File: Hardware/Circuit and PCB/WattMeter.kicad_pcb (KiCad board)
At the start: 2 copper layers, 185 x 126.1 mm, 80 parts, among them IC1 ATM90E32AS-AU-R, IC2 LM2621MMX_NOPB, J1 LCD Pins, J10 I2 Use/GND, J11 Input, J12 V3 Use/GND, J13 I1, J14 Series/Para, J15 Series/Para, J16 V2 Use/GND, J17 V1, J18 VCC Pins, J19 Boost Input, J2 Button Pins, J3 GSD09002SEU, J4 Extras, J5 SPI ATM90, J9 I3 Use/GND, T1 CT1020, T4 10:1, U1 ESP32-C6-DEVKITC-1-N8, U3 PCF8523T/1_118, Y1 16.384MHz, Y2 32.768kHz

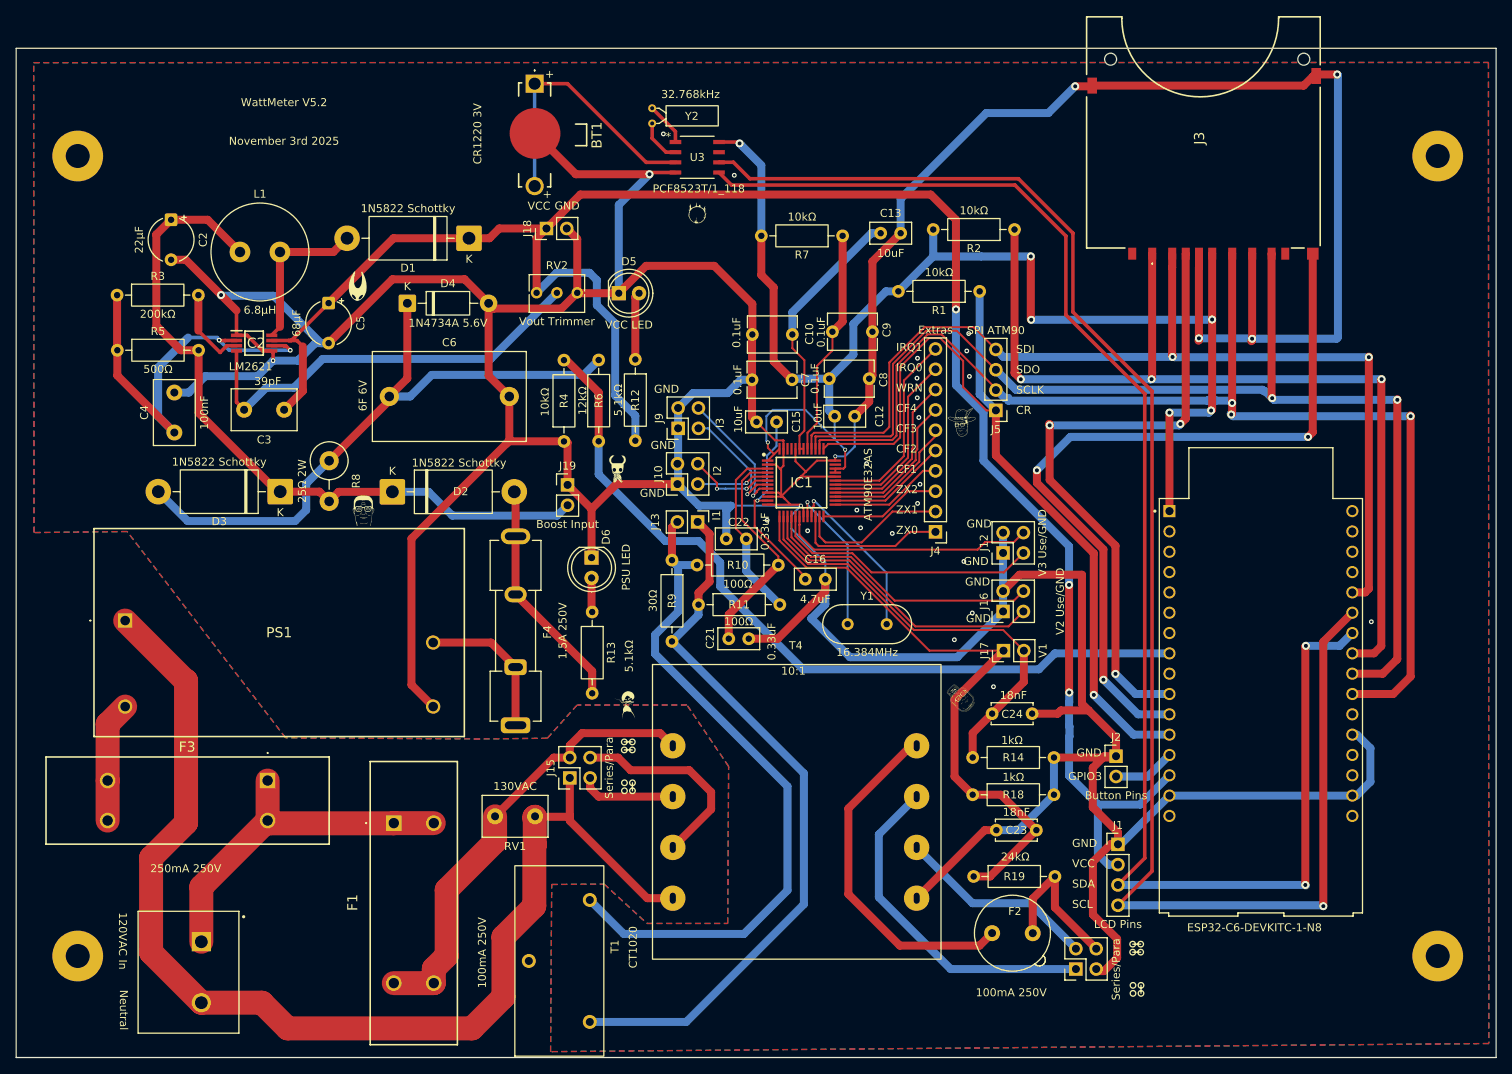
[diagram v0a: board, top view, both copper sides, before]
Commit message: Add some plots
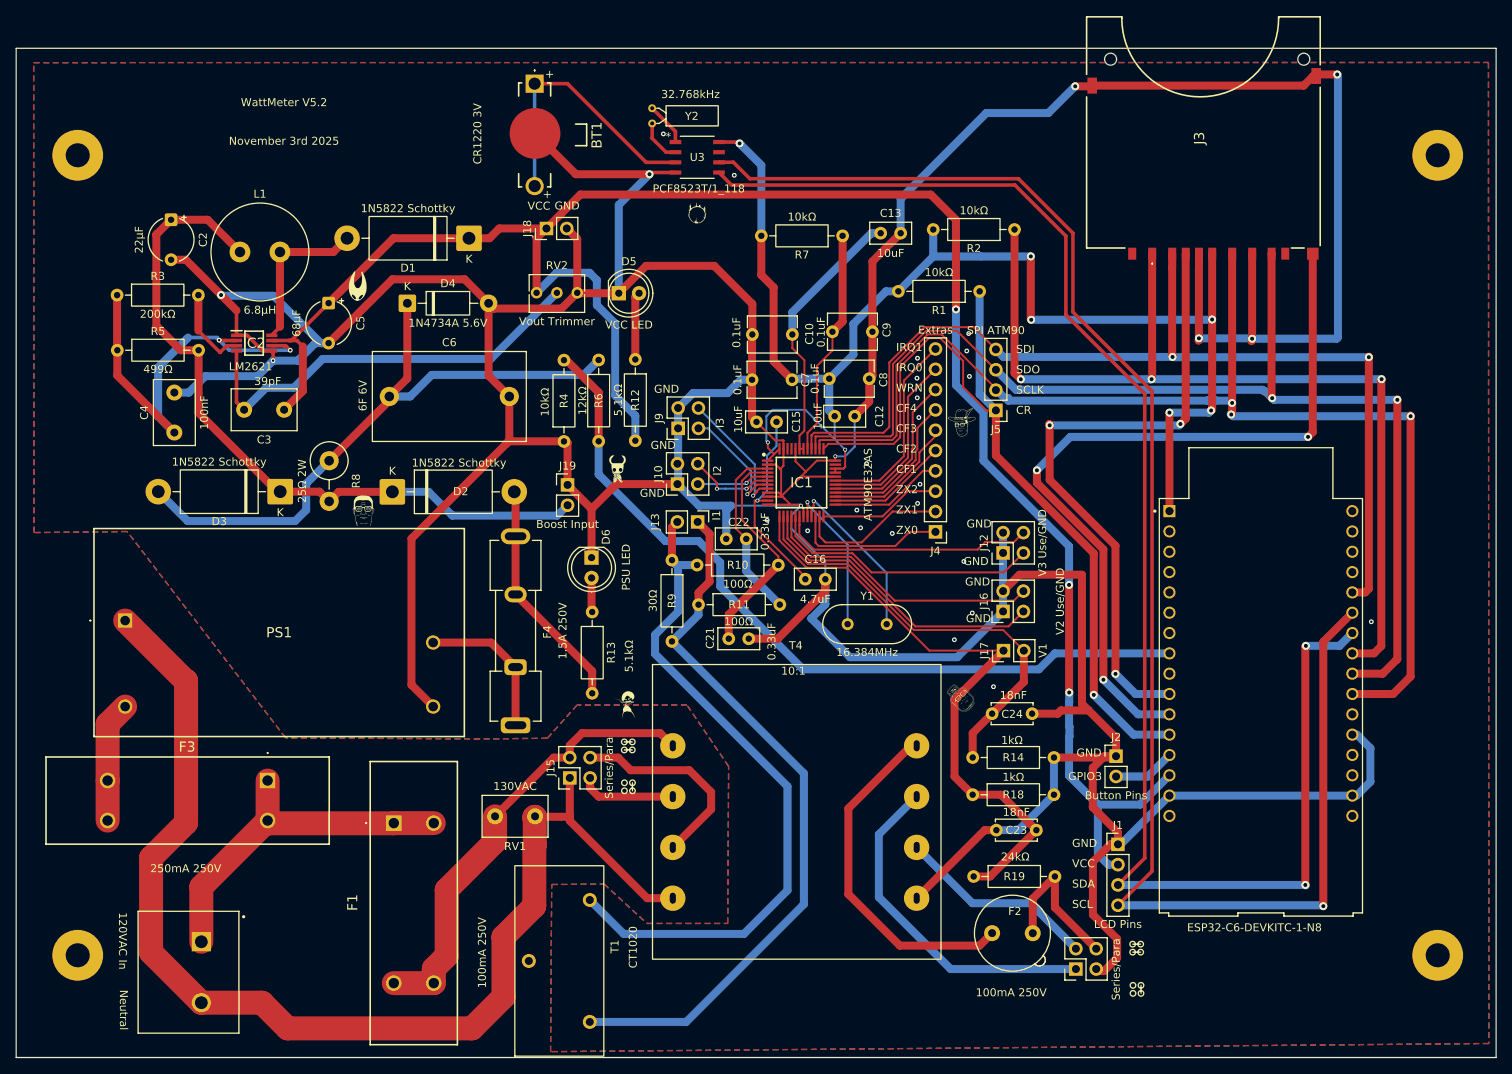
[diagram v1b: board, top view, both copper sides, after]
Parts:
- removed REF**: 1591XXF Enclosure 4 point, Mounting Footprints:1591XXF Enclosure 4 point
- added N1: Housing, Mounting Footprints:1591XXF Enclosure 4 point, F.Cu at (60.7, 50.4)
- R5: value 500Ω -> 499Ω
